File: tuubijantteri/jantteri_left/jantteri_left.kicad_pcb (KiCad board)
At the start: 2 copper layers, 61.5 x 61.5 mm, 56 parts, among them J1 Conn_02x08_Odd_Even, J2 Conn_01x03_Male, J3 Conn_02x03_Odd_Even, J4 DBG, J5 DBG, Q1 AO3400A, Q2 AO3401A, Q3 AO3400A, SW1 SW_Push, U1 AMS1117-3.3, U2 STM32L151C8TxA, U3 LM2596S-5, U4 W25Q128JVS, Y1 16MHz

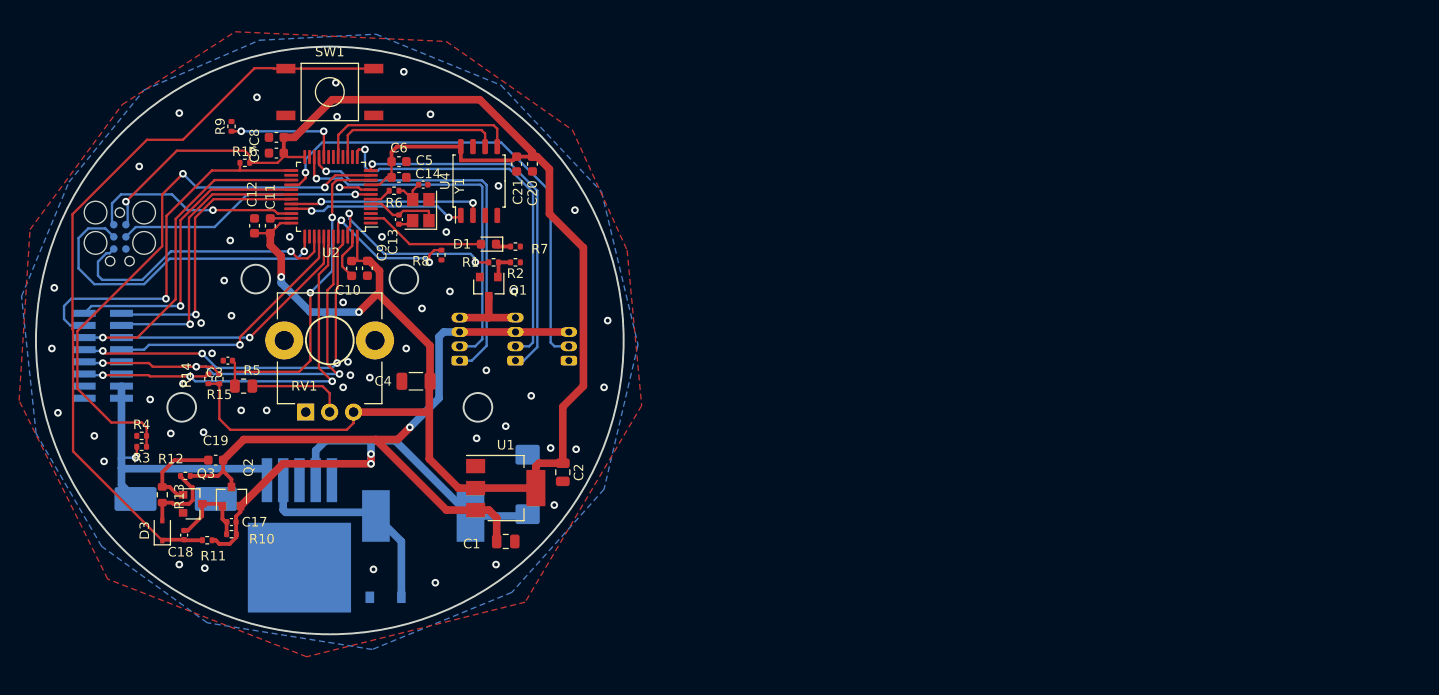
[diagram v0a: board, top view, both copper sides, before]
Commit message: update jantteri_right
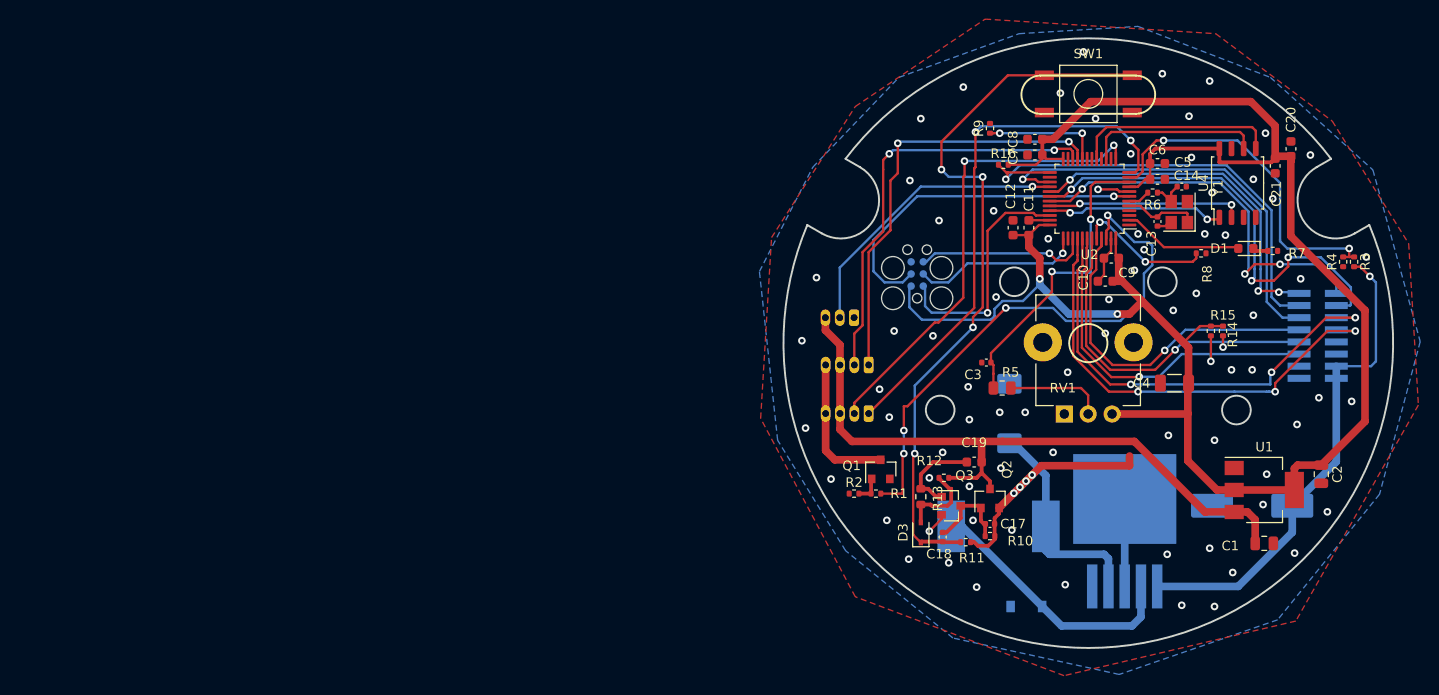
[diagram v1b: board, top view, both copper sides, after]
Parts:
- moved R3 128.3 mm to (188.3, 60.0), turned to 270 degrees
- moved J1 127.1 mm to (184.5, 67.8)
- moved R4 127.0 mm to (187.2, 60.0), turned to 90 degrees
- moved C15 112.7 mm to (177.7, 85.5), turned to 180 degrees
- moved R15 105.2 mm to (174.6, 67.3), turned to 90 degrees
- moved R14 105.0 mm to (173.4, 67.3), turned to 90 degrees
- moved U3 86.4 mm to (164.3, 88.2), turned to 90 degrees
- moved J3 83.5 mm to (142.6, 61.3), turned to 90 degrees
- moved R8 79.5 mm to (172.3, 59.1), turned to 0 degrees
- moved C20 79.4 mm to (181.7, 48.2), turned to 90 degrees
- moved C12 79.4 mm to (152.7, 56.4)
- moved C13 79.4 mm to (167.8, 55.8)
- moved C5 79.4 mm to (167.8, 51.4)
- moved C6 79.4 mm to (167.8, 49.7)
- moved R11 79.4 mm to (147.7, 89.4)
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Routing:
- net PERIPHERAL_EN: track 19.8 -> 56.8 mm, vias 2 -> 4
- net VIN_MEAS: track 58.9 -> 36.0 mm
- net STAT1_IN: track 27.4 -> 48.7 mm, vias 1 -> 3
- net STAT2_IN: track 27.2 -> 48.1 mm, vias 1 -> 3
- net V_SYSTEM_IN: track 31.7 -> 51.4 mm
- net LED: track 50.1 -> 30.7 mm
- net /STM32L151C8T6A/PA2: track 38.4 -> 55.9 mm, vias 1 -> 2
- net TXD_IN: track 30.2 -> 47.7 mm, vias 1 -> 3
- net /STM32L151C8T6A/SWCLK: track 34.9 -> 17.8 mm
- net +3V3: track 210.9 -> 197.4 mm, vias 3 -> 2
- net RXD_IN: track 28.9 -> 41.5 mm, vias 1 -> 3
- net GND: track 12.1 -> 23.8 mm, vias 52 -> 75
- net /STM32L151C8T6A/SWO: track 29.9 -> 18.2 mm
- net MOTOR_A_OUT: track 33.4 -> 44.2 mm
- net DRV_n_FAULT_OUT: track 39.3 -> 49.2 mm
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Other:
- board size 61.5 x 61.5 mm -> 63.8 x 63.8 mm

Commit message: Update projects
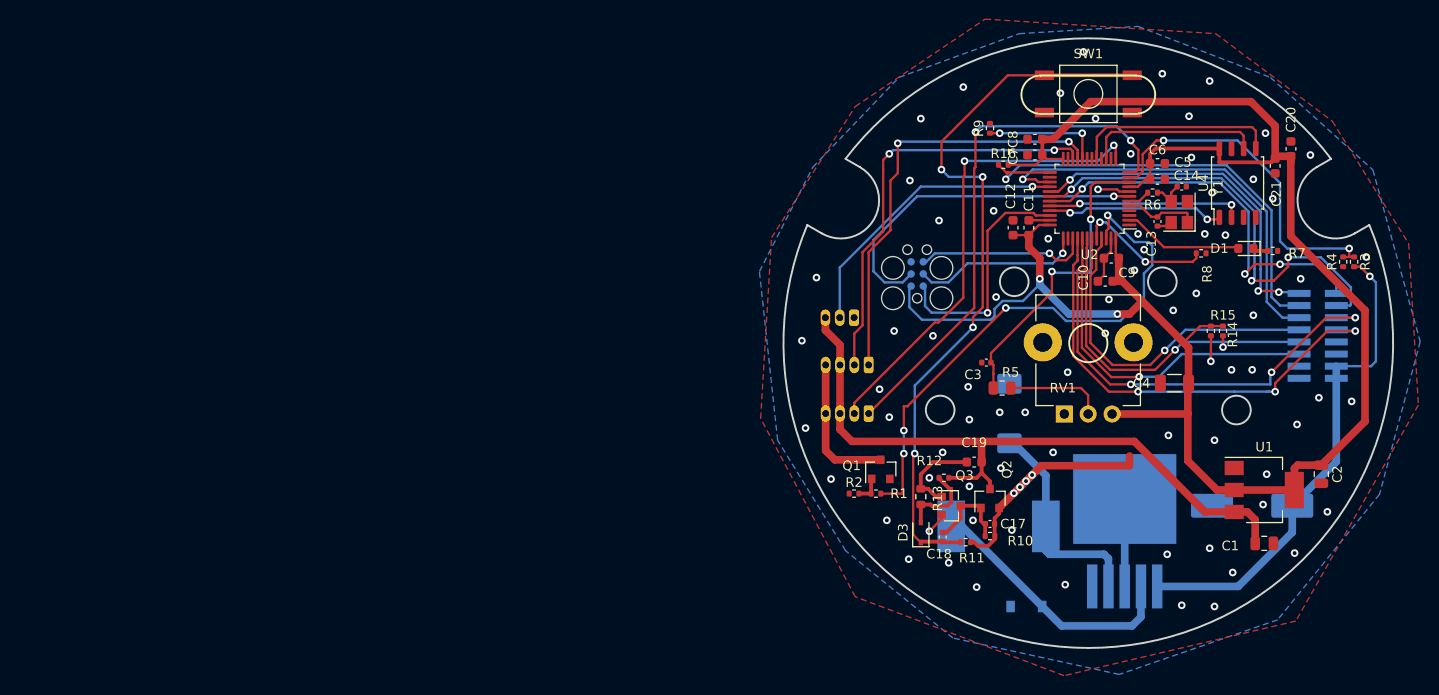
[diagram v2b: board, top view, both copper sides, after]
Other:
- net class Default removed
